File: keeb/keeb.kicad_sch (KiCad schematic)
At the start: 162 parts, among them J101 AVR-ISP-6, J102 USB_C_Receptacle_USB2.0, SW101 SW_Push, SW102 SW_Push, SW103 SW_Push, SW104 SW_Push, SW105 SW_Push, SW106 SW_Push, SW107 SW_Push, SW108 SW_Push, SW109 SW_Push, SW110 SW_Push, SW111 SW_Push, SW112 SW_Push, SW113 SW_Push, SW114 SW_Push, SW115 SW_Push, SW116 SW_Push, SW117 SW_Push, SW118 SW_Push, SW119 SW_Push, SW120 SW_Push, SW121 SW_Push, SW122 SW_Push, SW123 SW_Push, SW124 SW_Push, SW125 SW_Push, SW126 SW_Push, SW127 SW_Push, SW128 SW_Push, SW129 SW_Push, SW130 SW_Push, SW131 SW_Push, SW132 SW_Push, SW133 SW_Push, SW134 SW_Push, SW135 SW_Push, SW136 SW_Push, SW137 SW_Push, SW138 SW_Push, SW139 SW_Push, SW140 SW_Push, SW141 SW_Push, SW142 SW_Push, SW143 SW_Push, SW144 SW_Push, SW145 SW_Push, SW146 SW_Push, SW147 SW_Push, SW148 SW_Push, SW149 SW_Push, SW150 SW_Push, SW151 SW_Push, SW152 SW_Push, SW153 SW_Push, SW154 SW_Push, SW155 SW_Push, SW156 SW_Push, SW157 SW_Push, SW158 SW_Push, SW159 SW_Push, SW160 SW_Push, SW161 SW_Push, SW162 SW_Push, SW163 SW_Push, SW164 SW_Push, SW165 SW_Push, SW166 SW_Push, SW167 SW_Push, U101 TPD2S017, U102 ATmega32U4-MU, Y101 16Mhz

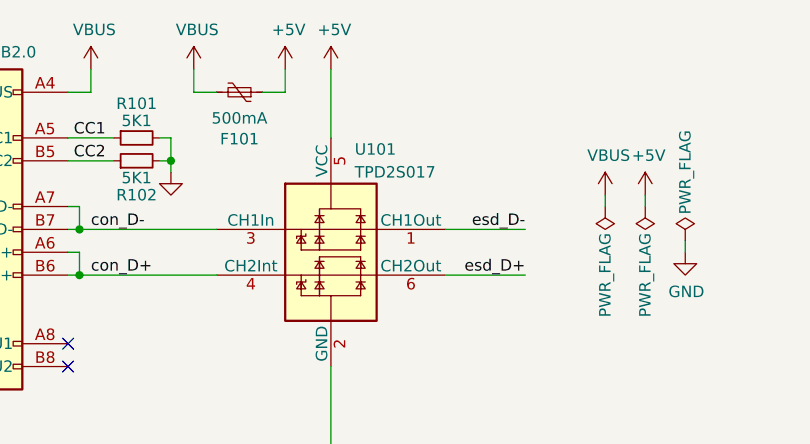
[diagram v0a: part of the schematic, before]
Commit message: all FP cleaned up and updated
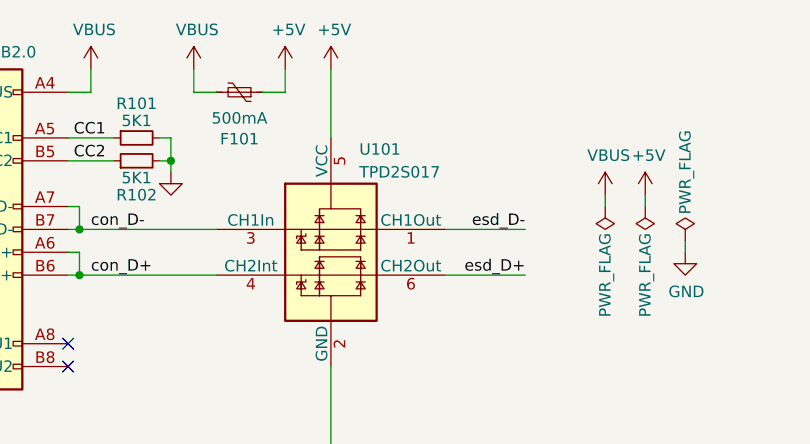
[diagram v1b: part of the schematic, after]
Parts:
- C101, C107: footprint Capacitor_SMD:C_0603_1608Metric -> unORTHOdox:C_0603_1608Metric
- C102, C103, C104, C105, C106, C108, C109: footprint Capacitor_SMD:C_0402_1005Metric -> unORTHOdox:C_0402_1005Metric
- D101, D102, D103, D104, D105, D106, D107, D108, D109, D110, D111, D112, D113, D114, D115, D116, D117, D118, D119, D120, D121, D122, D123, D124, D125, D126, D127, D128, D129, D130, D131, D132, D133, D134, D135, D136, D137, D138, D139, D140, D141, D142, D143, D144, D145, D146, D147, D148, D149, D150, D151, D152, D153, D154, D155, D156, D157, D158, D159, D160, D161, D162, D163, D164, D165, D166: footprint Diode_SMD:D_SOD-123F -> unORTHOdox:D_SOD-123F
- F101: footprint Fuse:Fuse_0603_1608Metric -> unORTHOdox:Fuse_0603_1608Metric
- R101, R102, R103, R104, R105, R106, R107, R108, R109, R110: footprint Resistor_SMD:R_0402_1005Metric -> unORTHOdox:R_0402_1005Metric
- SW167: footprint Button_Switch_SMD:SW_SPST_B3U-1000P -> unORTHOdox:SW_SPST_B3U-1000P
- U101: footprint Package_TO_SOT_SMD:SOT-23-6 -> unORTHOdox:SOT-23-6
- Y101: footprint Crystal:Crystal_SMD_2016-4Pin_2.0x1.6mm -> unORTHOdox:Crystal_SMD_2016-4Pin_2.0x1.6mm
